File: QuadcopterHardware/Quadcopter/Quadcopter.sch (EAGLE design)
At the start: 13 parts, among them M1 WIRELESS-NRF24L01, U1 ATMEGA328P_TQFP, U2 TC1262-3.3VDB

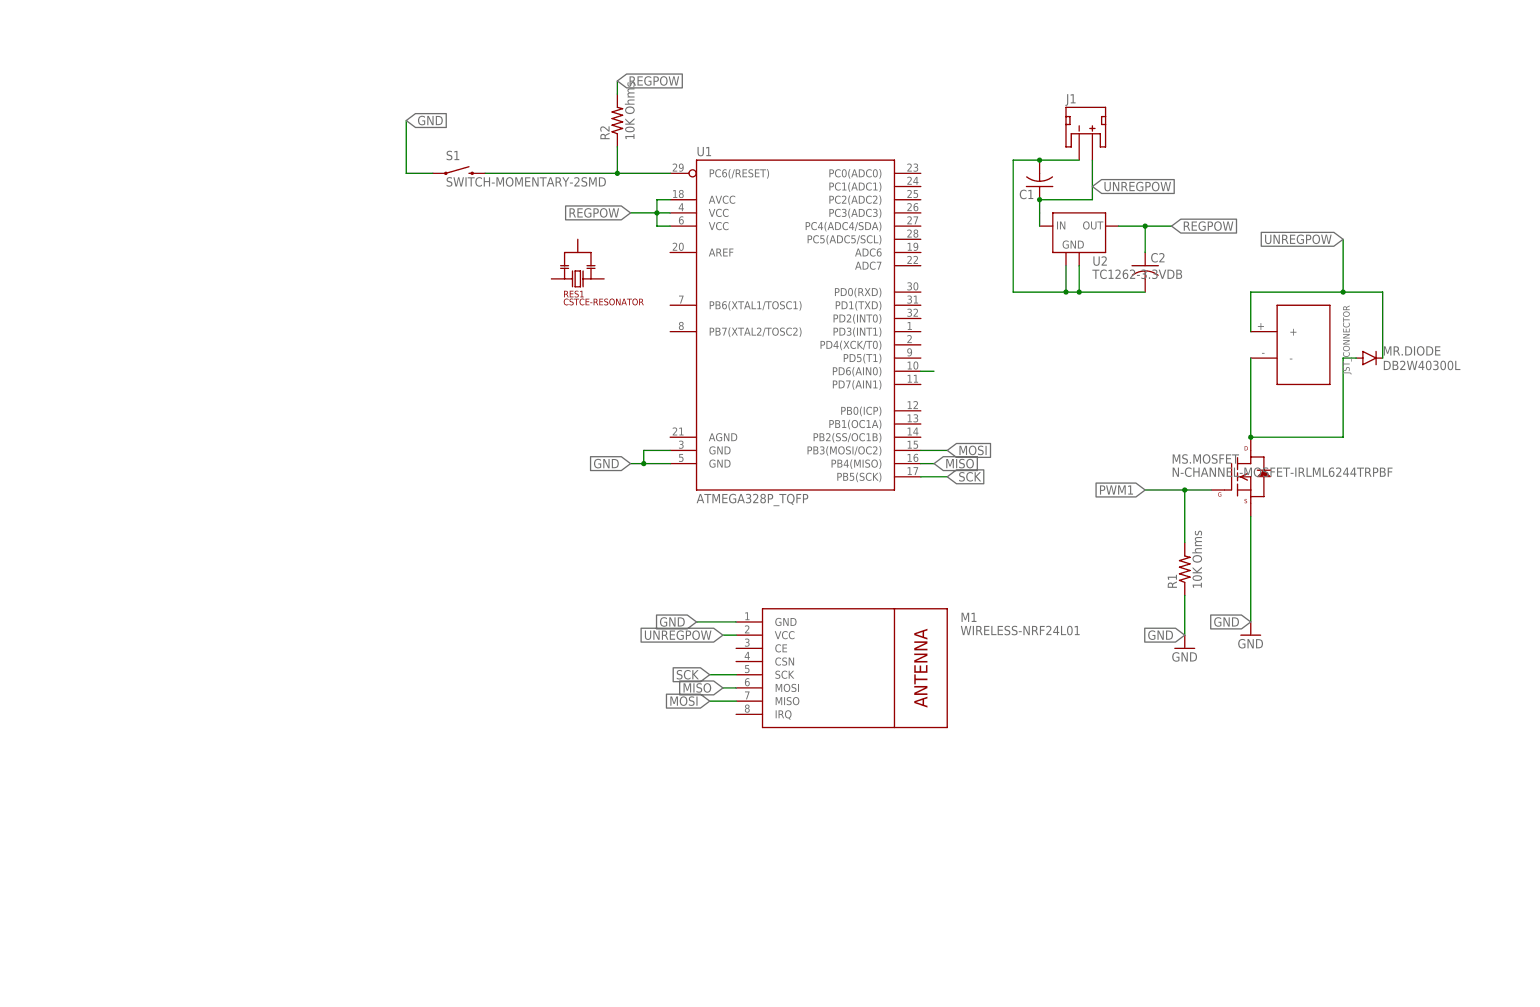
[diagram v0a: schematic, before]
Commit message: added to schematic...almost done :)
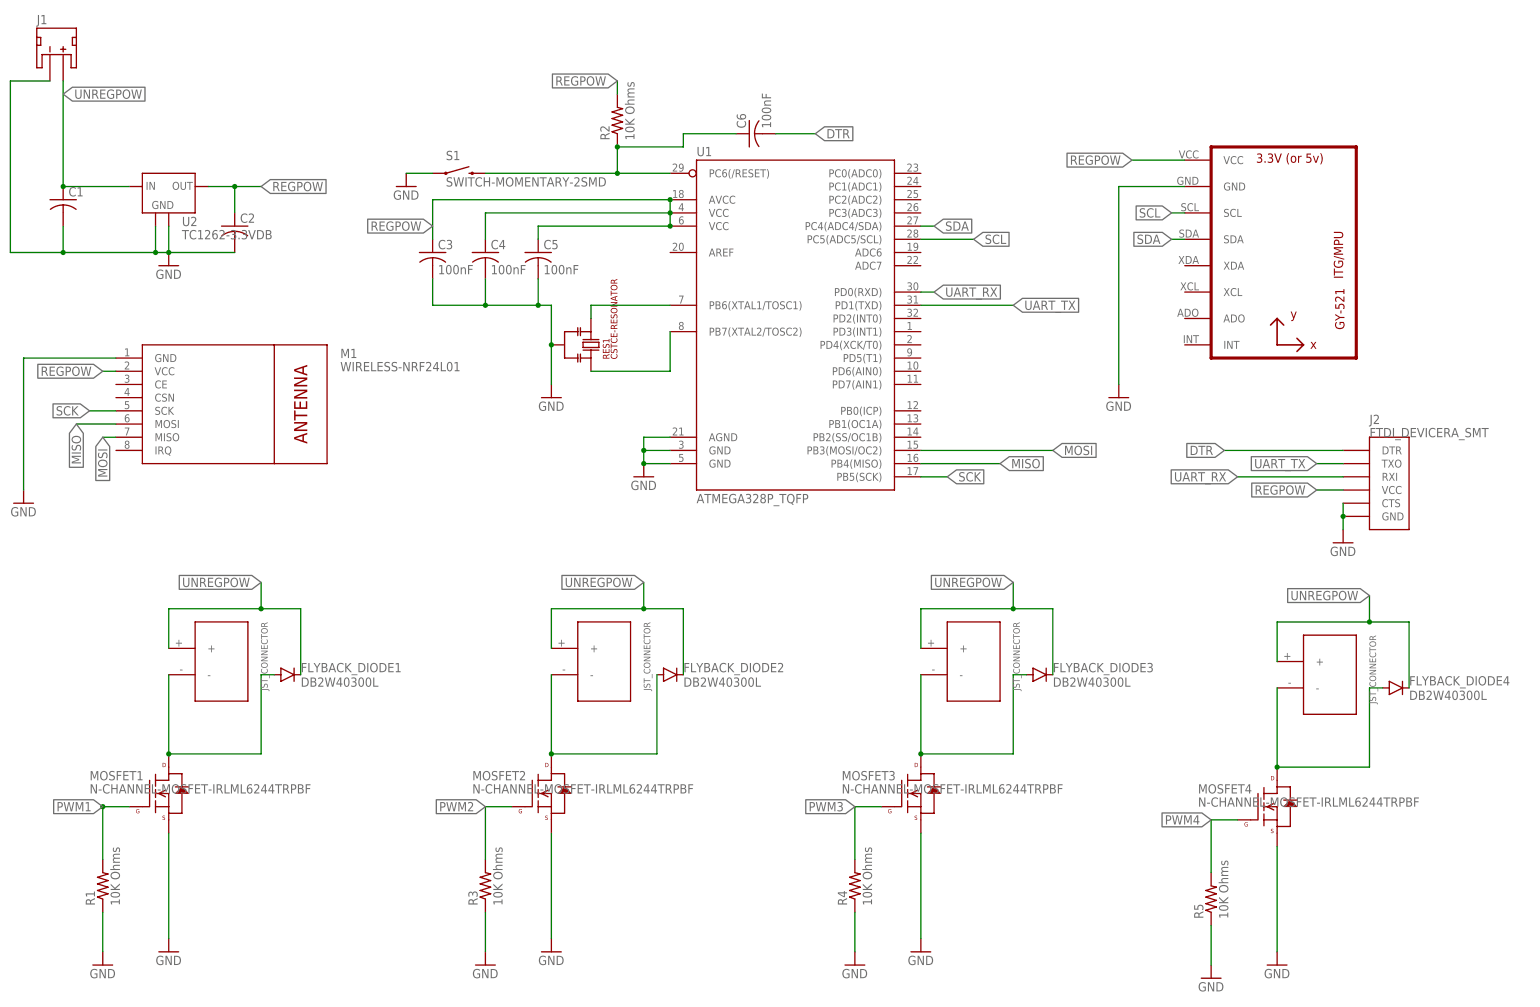
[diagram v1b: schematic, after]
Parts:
- removed MR.DIODE: DB2W40300L, quad:DB2W40300L
- removed MS.MOSFET: N-CHANNEL-MOSFET-IRLML6244TRPBF, quad:N-CHANNEL-MOSFET-IRLML6244TRPBF
- added C3, C4, C5, C6: 100nF, rcl:C-USC0603
- added FLYBACK_DIODE1, FLYBACK_DIODE2, FLYBACK_DIODE3, FLYBACK_DIODE4: DB2W40300L, quad:DB2W40300L
- added J2: FTDI_DEVICERA_SMT, quad:FTDI_DEVICERA_SMT
- added MOSFET1, MOSFET2, MOSFET3, MOSFET4: N-CHANNEL-MOSFET-IRLML6244TRPBF, quad:N-CHANNEL-MOSFET-IRLML6244TRPBF
- added MOTOR1, MOTOR2, MOTOR3: JST_CONNECTOR_FEMALE, quad:JST_CONNECTOR_FEMALE
- added R3, R4, R5: 10K Ohms, rcl:R-US_0204/5
- added U3: GY-521MPU6050, quad:GY-521MPU6050
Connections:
- removed net DRAIN: MOTOR.-, MR.DIODE.PPIN, MS.MOSFET.D
- removed net N$1: R2.1, S1.2, U1.PC6(/RESET)
- removed net N$3: U1.PD6(AIN0)
- new net DRAIN1: FLYBACK_DIODE1.PPIN, MOSFET1.D, MOTOR.-
- new net DRAIN2: FLYBACK_DIODE2.PPIN, MOSFET2.D, MOTOR1.-
- new net DRAIN3: FLYBACK_DIODE3.PPIN, MOSFET3.D, MOTOR2.-
- new net DRAIN4: FLYBACK_DIODE4.PPIN, MOSFET4.D, MOTOR3.-
- new net DTR: C6.2, J2.DTR
- new net PWM2: MOSFET2.G, R3.2
- new net PWM3: MOSFET3.G, R4.2
- new net PWM4: MOSFET4.G, R5.2
- new net RST: C6.1, R2.1, S1.2, U1.PC6(/RESET)
- new net SCL: U1.PC5(ADC5/SCL), U3.SCL
- new net SDA: U1.PC4(ADC4/SDA), U3.SDA
- new net UART_RX: J2.RXI, U1.PD0(RXD)
- new net UART_TX: J2.TXO, U1.PD1(TXD)
- new net XTAL1: RES1.P$3, U1.PB6(XTAL1/TOSC1)
- new net XTAL2: RES1.P$1, U1.PB7(XTAL2/TOSC2)
- net GND: now also C3.2, C4.2, C5.2, J2.CTS, J2.GND, MOSFET1.S, MOSFET2.S, MOSFET3.S, MOSFET4.S, R3.1, R4.1, R5.1, RES1.P$2, U1.AGND, U3.GND; no longer MS.MOSFET.S
- net PWM1: now also MOSFET1.G; no longer MS.MOSFET.G
- net REGPOW: now also C3.1, C4.1, C5.1, J2.VCC, M1.VCC, U3.VCC
- net UNREGPOW: now also FLYBACK_DIODE1.GPIN, FLYBACK_DIODE2.GPIN, FLYBACK_DIODE3.GPIN, FLYBACK_DIODE4.GPIN, MOTOR1.+, MOTOR2.+, MOTOR3.+; no longer M1.VCC, MR.DIODE.GPIN
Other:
- moved on the sheet: C1, C2, J1, M1, R1, RES1, U2
